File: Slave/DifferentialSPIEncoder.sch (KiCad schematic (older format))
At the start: 24 parts, among them J1 Conn_01x05_Male, J2 8P8C_Shielded, U2 AS5048A, U3 MAX485E, U4 MAX485E, U5 MAX485E

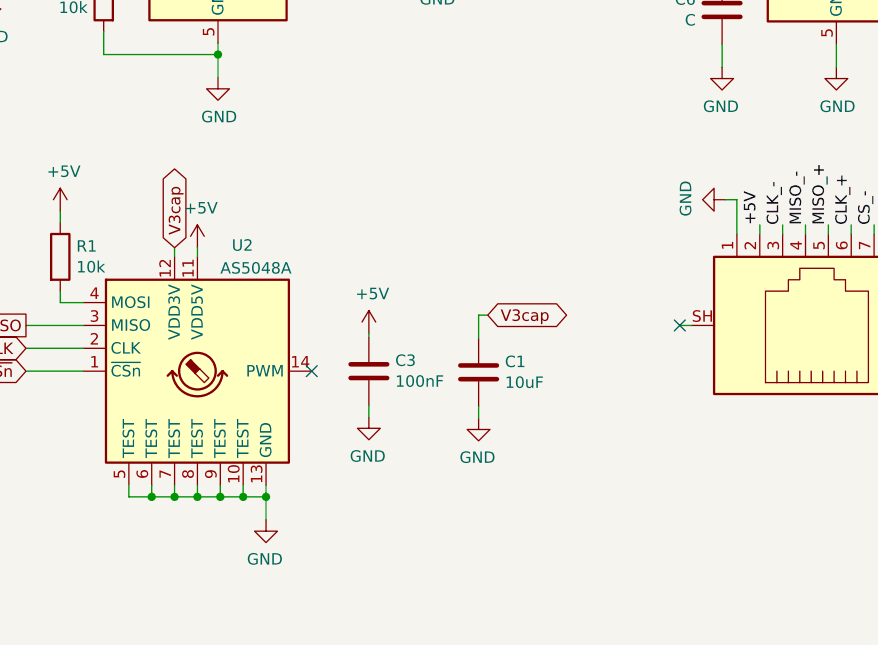
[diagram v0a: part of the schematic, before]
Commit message: Shame. Shame. Shame.
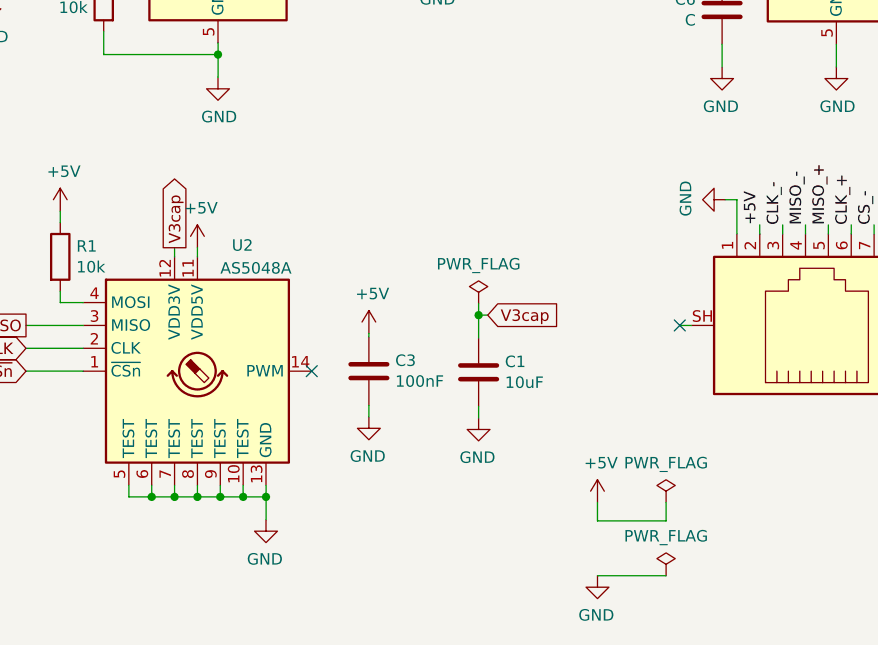
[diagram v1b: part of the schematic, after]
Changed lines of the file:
@@
 Wire Wire Line
 	3910 3360 3860 3360
-Text GLabel 3020 3315 2    50   BiDi ~ 0
+Text GLabel 3020 3315 2    50   Input ~ 0
 V3cap
 Connection ~ 1840 925
@@
 Wire Wire Line
 	1650 3060 1650 3020
-Text GLabel 1650 3020 1    50   BiDi ~ 0
+Text GLabel 1650 3020 1    50   Output ~ 0
 V3cap
 $Comp
@@
 	2500 3395 2500 3410
 $Comp
-L power:+5V #PWR?
+L power:+5V #PWR0108
 U 1 1 5DAC799E
 P 1750 3020
-F 0 "#PWR?" H 1750 2870 50  0001 C CNN
+F 0 "#PWR0108" H 1750 2870 50  0001 C CNN
 F 1 "+5V" H 1765 3193 50  0000 C CNN
 F 2 "" H 1750 3020 50  0001 C CNN
@@
 	1    0    0    -1
 $EndComp
+$Comp
+L power:+5V #PWR0109
+U 1 1 5E22FEAE
+P 3500 4135
+F 0 "#PWR0109" H 3500 3985 50  0001 C CNN
+F 1 "+5V" H 3515 4308 50  0000 C CNN
+F 2 "" H 3500 4135 50  0001 C CNN
+F 3 "" H 3500 4135 50  0001 C CNN
+	1    3500 4135
+	1    0    0    -1
+$EndComp
+$Comp
+L power:GND #PWR0110
+U 1 1 5E233C39
+P 3500 4455
+F 0 "#PWR0110" H 3500 4205 50  0001 C CNN
+F 1 "GND" H 3505 4282 50  0000 C CNN
+F 2 "" H 3500 4455 50  0001 C CNN
+F 3 "" H 3500 4455 50  0001 C CNN
+	1    3500 4455
+	-1   0    0    -1
+$EndComp
+$Comp
+L power:PWR_FLAG #FLG0101
+U 1 1 5E237BCC
+P 3800 4135
+F 0 "#FLG0101" H 3800 4210 50  0001 C CNN
+F 1 "PWR_FLAG" H 3800 4308 50  0000 C CNN
+F 2 "" H 3800 4135 50  0001 C CNN
+F 3 "~" H 3800 4135 50  0001 C CNN
+	1    3800 4135
+	1    0    0    -1
+$EndComp
+Wire Wire Line
+	3500 4135 3500 4215
+Wire Wire Line
+	3500 4215 3800 4215
+Wire Wire Line
+	3800 4215 3800 4135
+$Comp
+L power:PWR_FLAG #FLG0102
+U 1 1 5E23CAF5
+P 3800 4455
+F 0 "#FLG0102" H 3800 4530 50  0001 C CNN
+F 1 "PWR_FLAG" H 3800 4628 50  0000 C CNN
+F 2 "" H 3800 4455 50  0001 C CNN
+F 3 "~" H 3800 4455 50  0001 C CNN
+	1    3800 4455
+	1    0    0    -1
+$EndComp
+Wire Wire Line
+	3500 4455 3800 4455
+$Comp
+L power:PWR_FLAG #FLG0103
+U 1 1 5E251298
+P 2980 3265
+F 0 "#FLG0103" H 2980 3340 50  0001 C CNN
+F 1 "PWR_FLAG" H 2980 3438 50  0000 C CNN
+F 2 "" H 2980 3265 50  0001 C CNN
+F 3 "~" H 2980 3265 50  0001 C CNN
+	1    2980 3265
+	1    0    0    -1
+$EndComp
+Wire Wire Line
+	2980 3265 2980 3315
+Connection ~ 2980 3315
 $EndSCHEMATC
